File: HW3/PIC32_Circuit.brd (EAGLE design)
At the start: 50 x 50 mm, 22 parts, among them J3 USB-MB-H

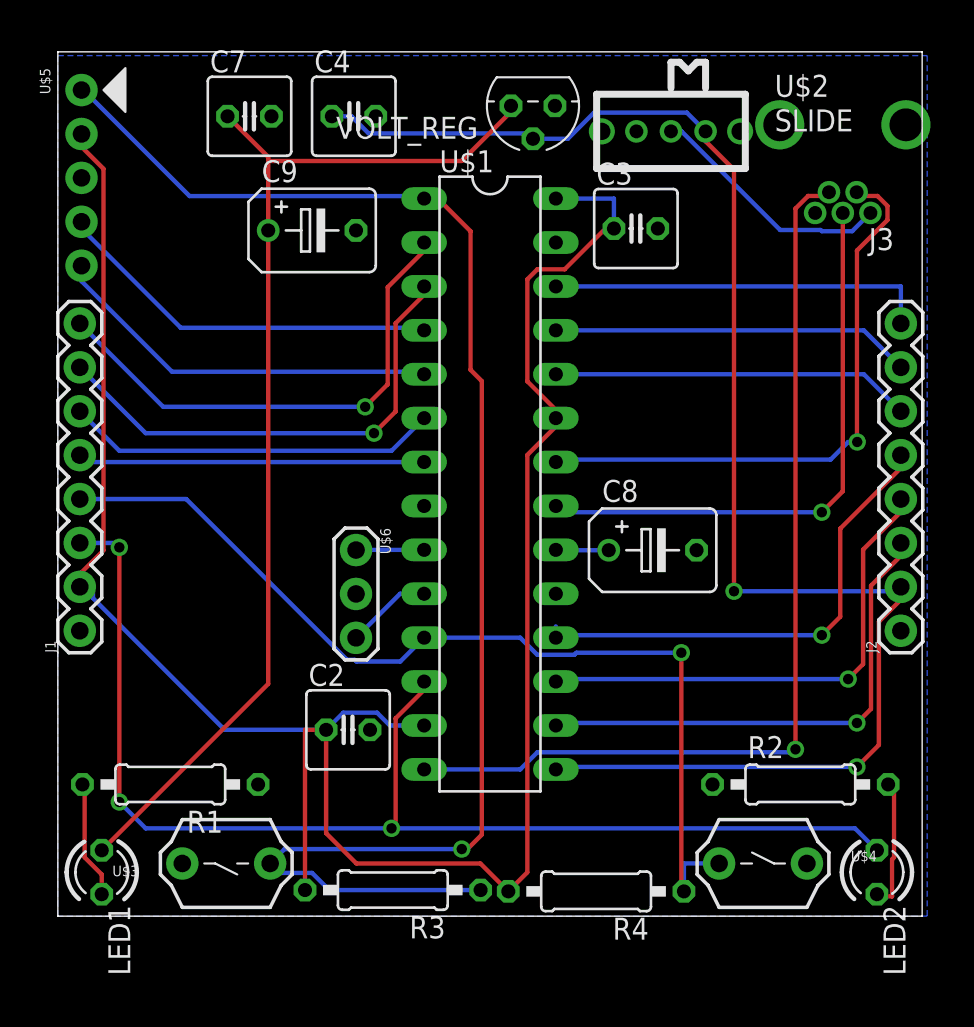
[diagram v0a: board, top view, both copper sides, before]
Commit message: Final Board
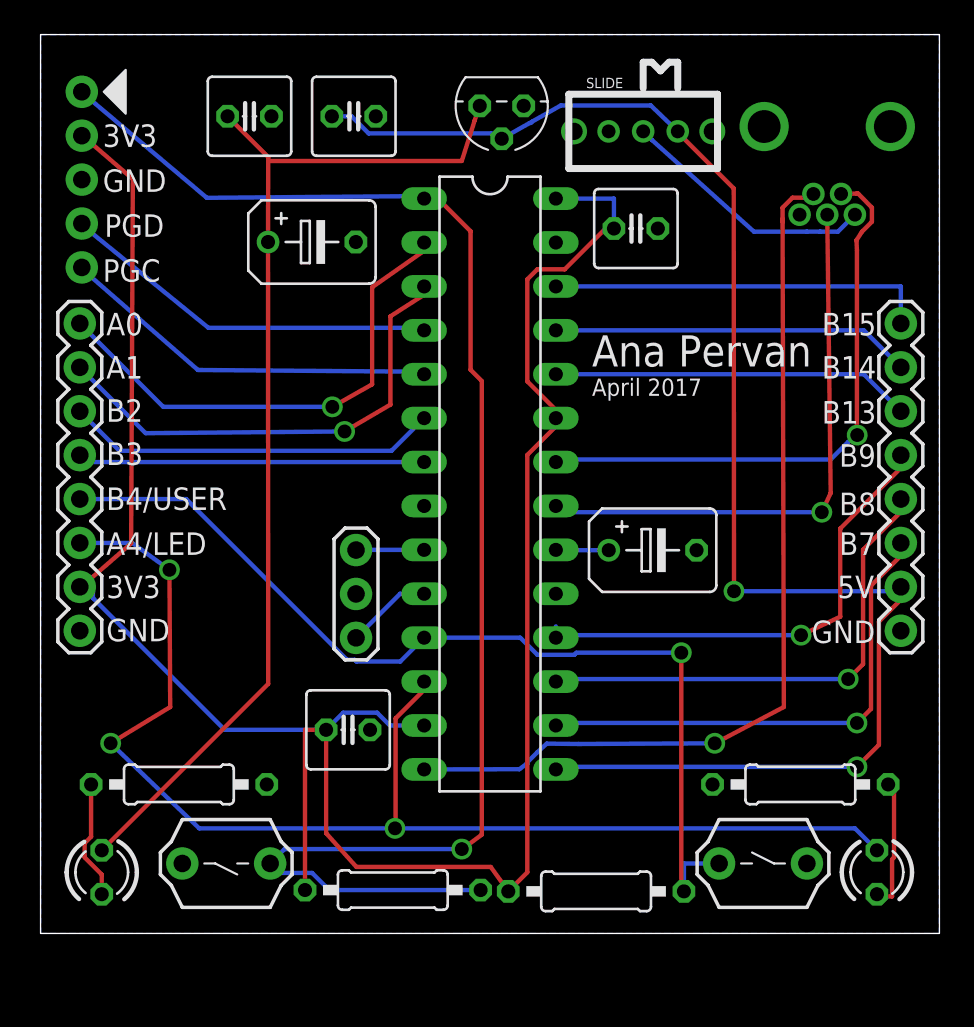
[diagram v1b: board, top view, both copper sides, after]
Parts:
- moved VOLT_REG 1.81 mm to (25.7, 46.9)
- moved U$2 1.61 mm to (33.9, 45.4)
- moved J3 0.91 mm to (44.5, 45.7)
- moved C9 0.67 mm to (14.7, 39.0)
- moved R1 0.50 mm to (7.00, 7.62)
- moved U$5 0.10 mm to (1.39, 47.7)
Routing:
- net USBID: track 55.6 -> 53.0 mm
- net A4/LED: track 71.4 -> 73.7 mm
- net +3V3: track 128.8 -> 130.6 mm
- net N$3: track 63.0 -> 62.0 mm
- net +5V: track 89.4 -> 88.4 mm
- net PGC: track 22.9 -> 22.1 mm
- net MCLR: track 87.3 -> 86.4 mm
- net PGD: track 22.7 -> 22.0 mm
- net VBUS: track 14.4 -> 14.9 mm
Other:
- board size 50 x 50 mm -> 52 x 52 mm
- board text added: "3V3"
- board text added: "5V"
- board text added: "A0"
- board text added: "A1"
- board text added: "A4/LED"
- board text added: "Ana Pervan"
- board text added: "April 2017"
- board text added: "B13"
- board text added: "B14"
- board text added: "B15"
- board text added: "B2"
- board text added: "B3"
- board text added: "B4/USER"
- board text added: "B7"
- board text added: "B8"
- board text added: "B9"
- board text added: "GND"
- board text added: "PGC"
- board text added: "PGD"
